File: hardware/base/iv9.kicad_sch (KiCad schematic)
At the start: 0 parts

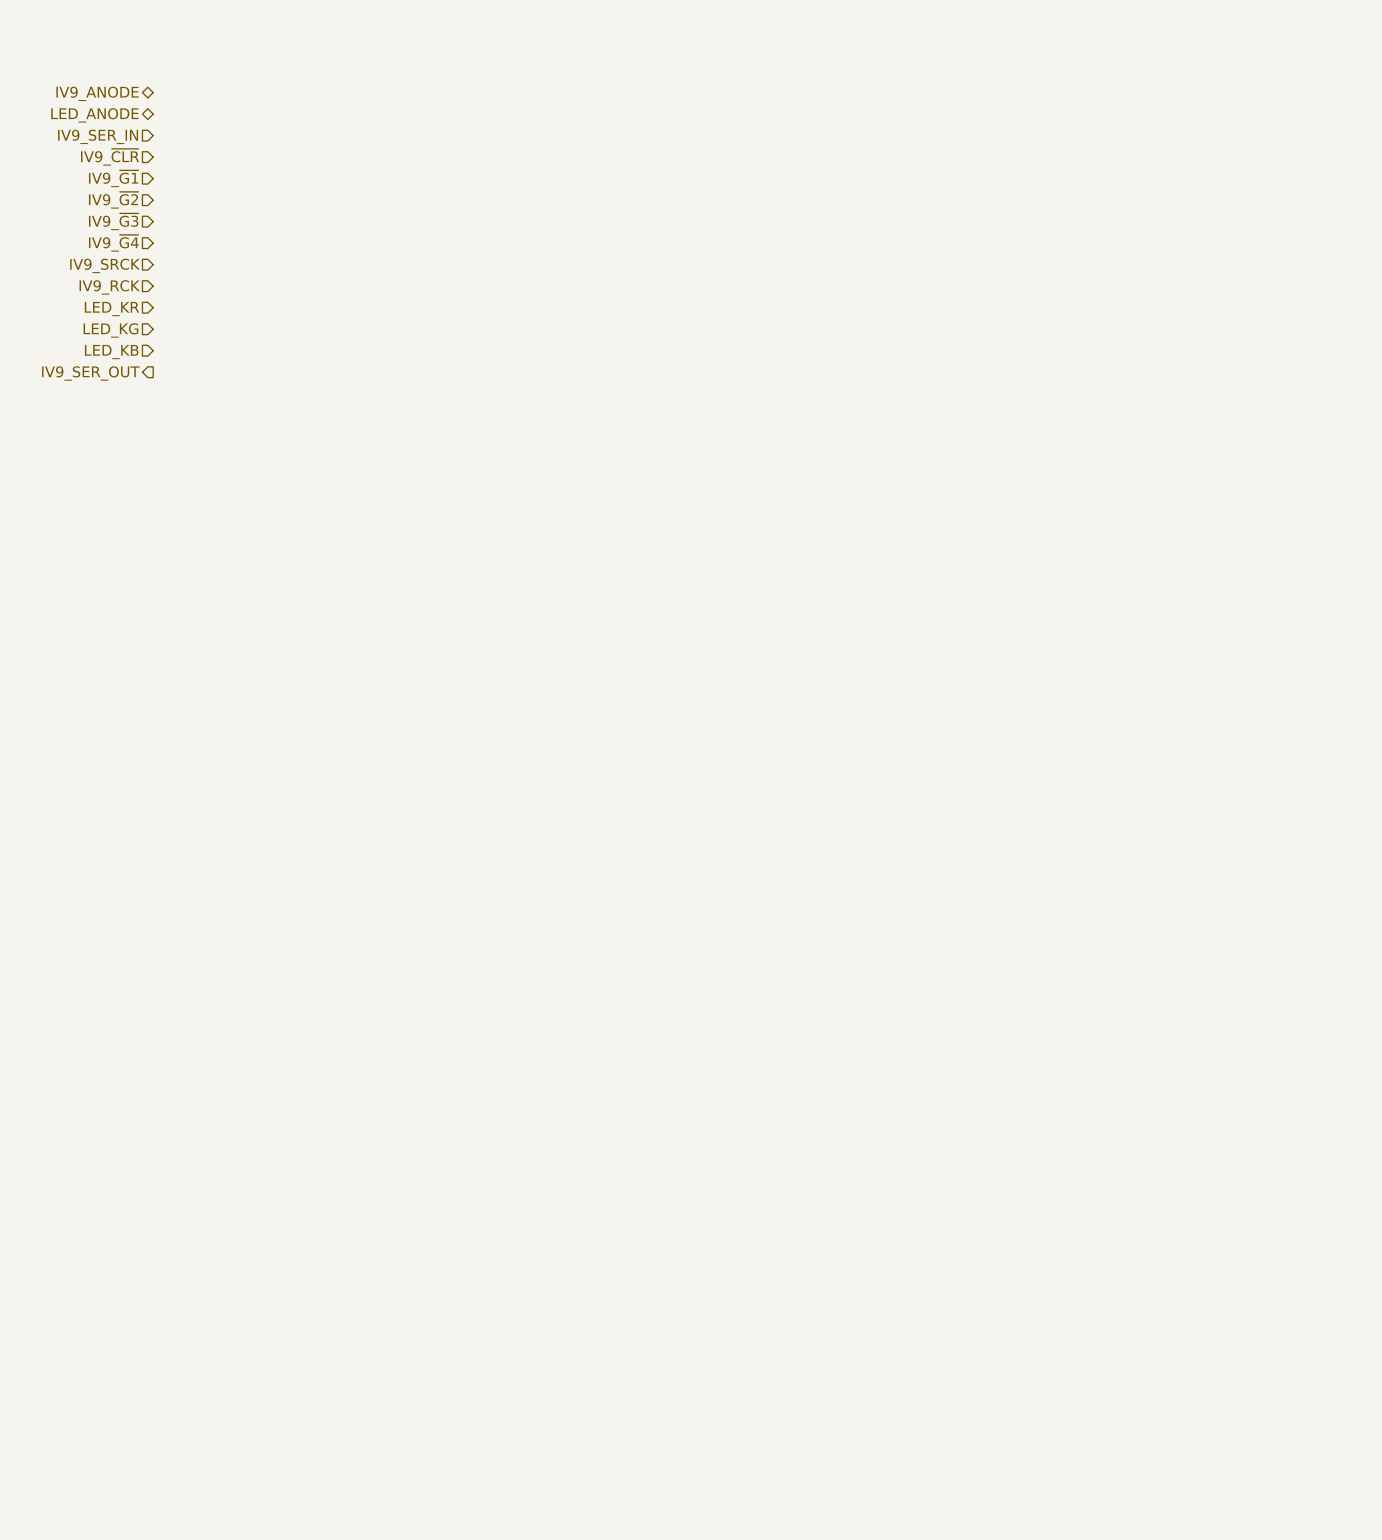
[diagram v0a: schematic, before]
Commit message: Base PCB WIP
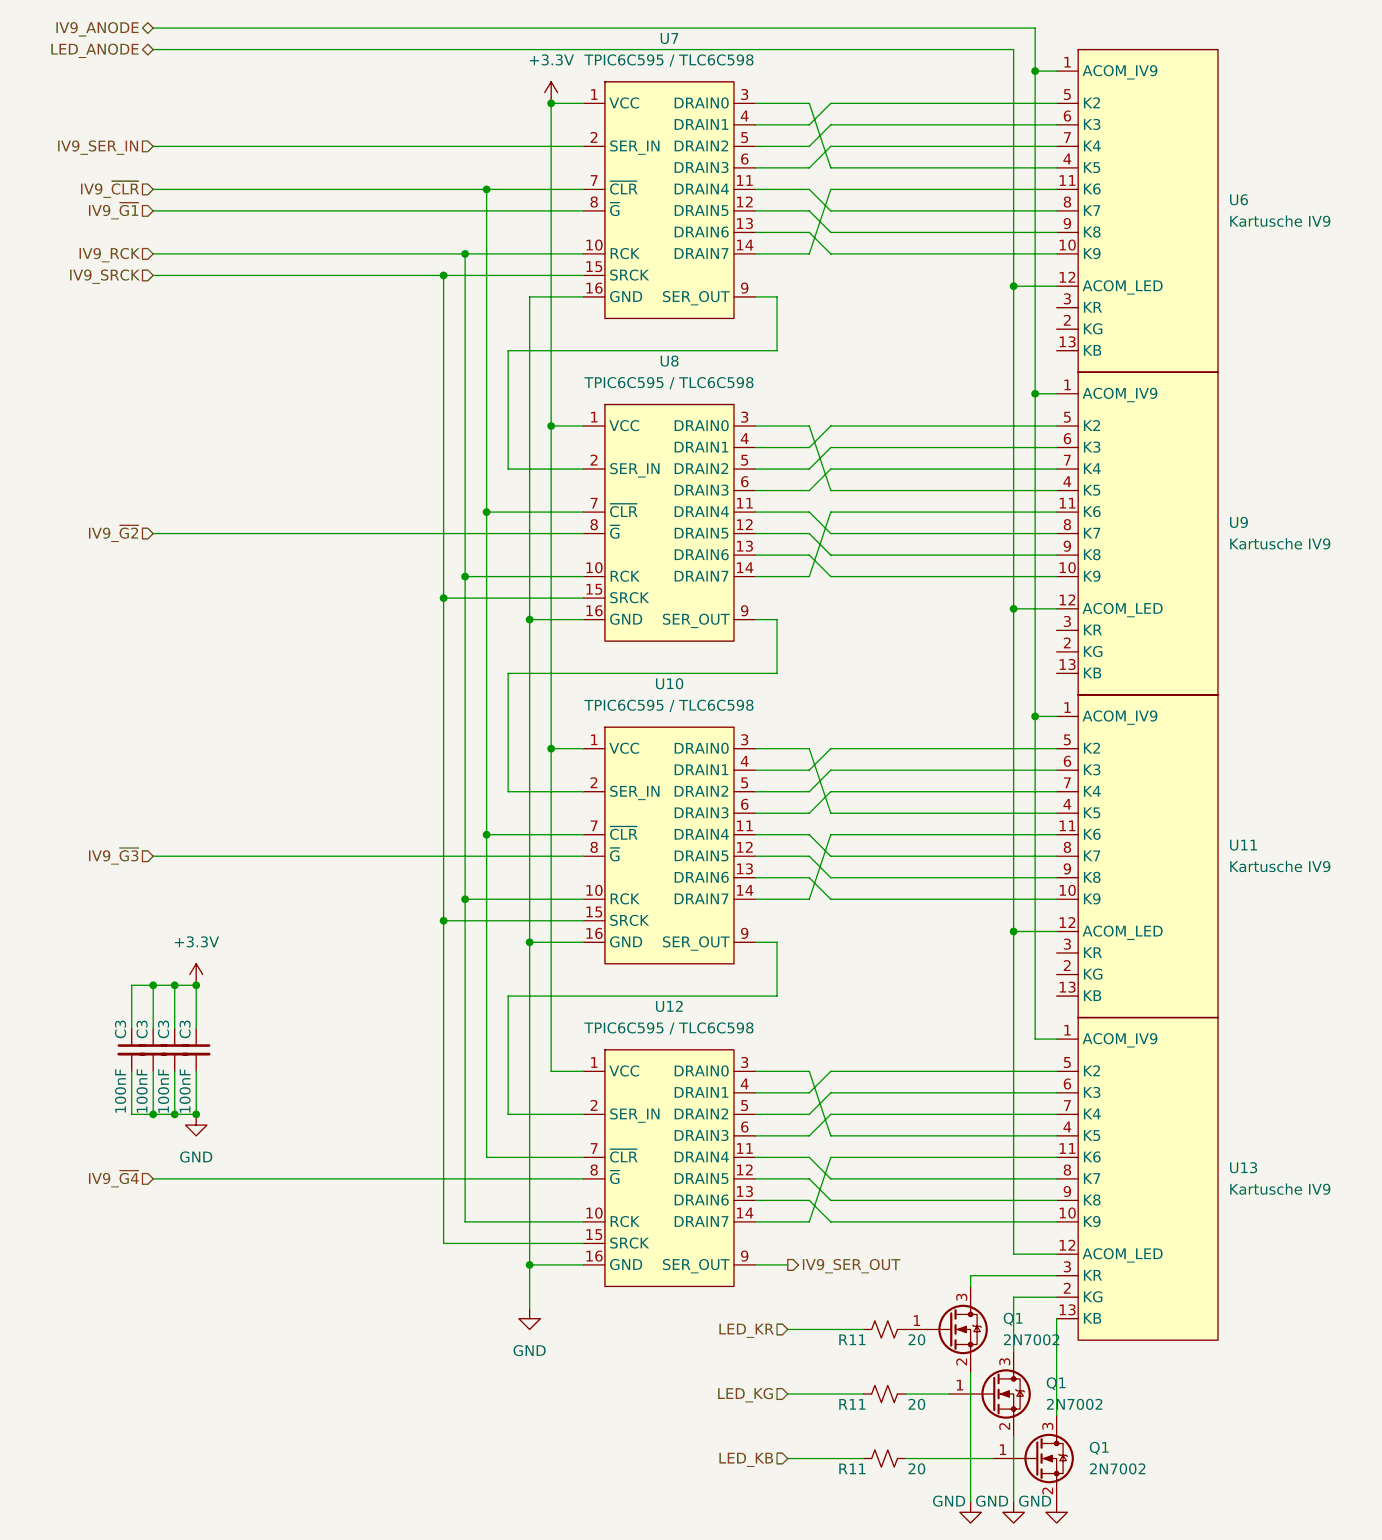
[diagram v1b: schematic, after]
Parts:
- added C3 (x4): 100nF, Capacitor_SMD:C_0402_1005Metric_Pad0.74x0.62mm_HandSolder, symbol Device:C_Small
- added Q1 (x3): 2N7002, Package_TO_SOT_SMD:SOT-23, symbol Transistor_FET:2N7002
- added R11 (x3): 20, Resistor_SMD:R_0402_1005Metric, symbol Device:R_Small_US
- added U10, U12, U7, U8: TPIC6C595 / TLC6C598, Package_SO:SOIC-16_3.9x9.9mm_P1.27mm, symbol Flora:TPIC6C595
- added U11, U13, U6, U9: Kartusche IV9, Flora:Kartusche_IV9, symbol Flora:Kartusche_IV9
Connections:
- net IV9_ANODE: now also U11.1 (ACOM_IV9), U11.14 (ACOM_IV9), U13.1 (ACOM_IV9), U13.14 (ACOM_IV9), U6.1 (ACOM_IV9), U6.14 (ACOM_IV9), U9.1 (ACOM_IV9), U9.14 (ACOM_IV9)
- net IV9_RCK: now also U10.10 (RCK), U12.10 (RCK), U7.10 (RCK), U8.10 (RCK)
- net IV9_SER_IN: now also U7.2 (SER_IN)
- net IV9_SER_OUT: now also U12.9 (SER_OUT)
- net IV9_SRCK: now also U10.15 (SRCK), U12.15 (SRCK), U7.15 (SRCK), U8.15 (SRCK)
- net IV9_~{CLR}: now also U10.7 (~{CLR}), U12.7 (~{CLR}), U7.7 (~{CLR}), U8.7 (~{CLR})
- net IV9_~{G1}: now also U7.8 (~{G})
- net IV9_~{G2}: now also U8.8 (~{G})
- net IV9_~{G3}: now also U10.8 (~{G})
- net IV9_~{G4}: now also U12.8 (~{G})
- net LED_ANODE: now also U11.12 (ACOM_LED), U13.12 (ACOM_LED), U6.12 (ACOM_LED), U9.12 (ACOM_LED)
- net LED_KB: now also R11.1
- net LED_KG: now also R11.1
- net LED_KR: now also R11.1
- new net: Q1.1 (G), R11.2 (x3)
- new net: U6.10 (K9), U7.13 (DRAIN6)
- new net: U6.11 (K6), U7.14 (DRAIN7)
- new net: U6.4 (K5), U7.3 (DRAIN0)
- new net: U6.5 (K2), U7.4 (DRAIN1)
- new net: U6.6 (K3), U7.5 (DRAIN2)
- new net: U6.7 (K4), U7.6 (DRAIN3)
- new net: U6.8 (K7), U7.11 (DRAIN4)
- new net: U6.9 (K8), U7.12 (DRAIN5)
- new net: U10.13 (DRAIN6), U11.10 (K9)
- new net: U10.14 (DRAIN7), U11.11 (K6)
- new net: U10.3 (DRAIN0), U11.4 (K5)
- new net: U10.4 (DRAIN1), U11.5 (K2)
- new net: U10.5 (DRAIN2), U11.6 (K3)
- new net: U10.6 (DRAIN3), U11.7 (K4)
- new net: U10.11 (DRAIN4), U11.8 (K7)
- new net: U10.12 (DRAIN5), U11.9 (K8)
- new net: Q1.3 (D), U13.2 (KG)
- new net: U10.2 (SER_IN), U8.9 (SER_OUT)
- new net: U10.9 (SER_OUT), U12.2 (SER_IN)
- new net: Q1.3 (D), U13.3 (KR)
- new net: U12.13 (DRAIN6), U13.10 (K9)
- new net: U12.14 (DRAIN7), U13.11 (K6)
- new net: Q1.3 (D), U13.13 (KB)
- new net: U12.3 (DRAIN0), U13.4 (K5)
- new net: U12.4 (DRAIN1), U13.5 (K2)
- new net: U12.5 (DRAIN2), U13.6 (K3)
- new net: U12.6 (DRAIN3), U13.7 (K4)
- new net: U12.11 (DRAIN4), U13.8 (K7)
- new net: U12.12 (DRAIN5), U13.9 (K8)
- new net: U7.9 (SER_OUT), U8.2 (SER_IN)
- new net: U8.13 (DRAIN6), U9.10 (K9)
- new net: U8.14 (DRAIN7), U9.11 (K6)
- new net: U8.3 (DRAIN0), U9.4 (K5)
- new net: U8.4 (DRAIN1), U9.5 (K2)
- new net: U8.5 (DRAIN2), U9.6 (K3)
- new net: U8.6 (DRAIN3), U9.7 (K4)
- new net: U8.11 (DRAIN4), U9.8 (K7)
- new net: U8.12 (DRAIN5), U9.9 (K8)
- new net +3.3V: C3.1, C3.1, C3.1, C3.1, U10.1 (VCC), U12.1 (VCC), U7.1 (VCC), U8.1 (VCC)
- new net GND: C3.2, C3.2, C3.2, C3.2, Q1.2 (S), Q1.2 (S), Q1.2 (S), U10.16 (GND), U12.16 (GND), U7.16 (GND), U8.16 (GND)

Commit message: Minor
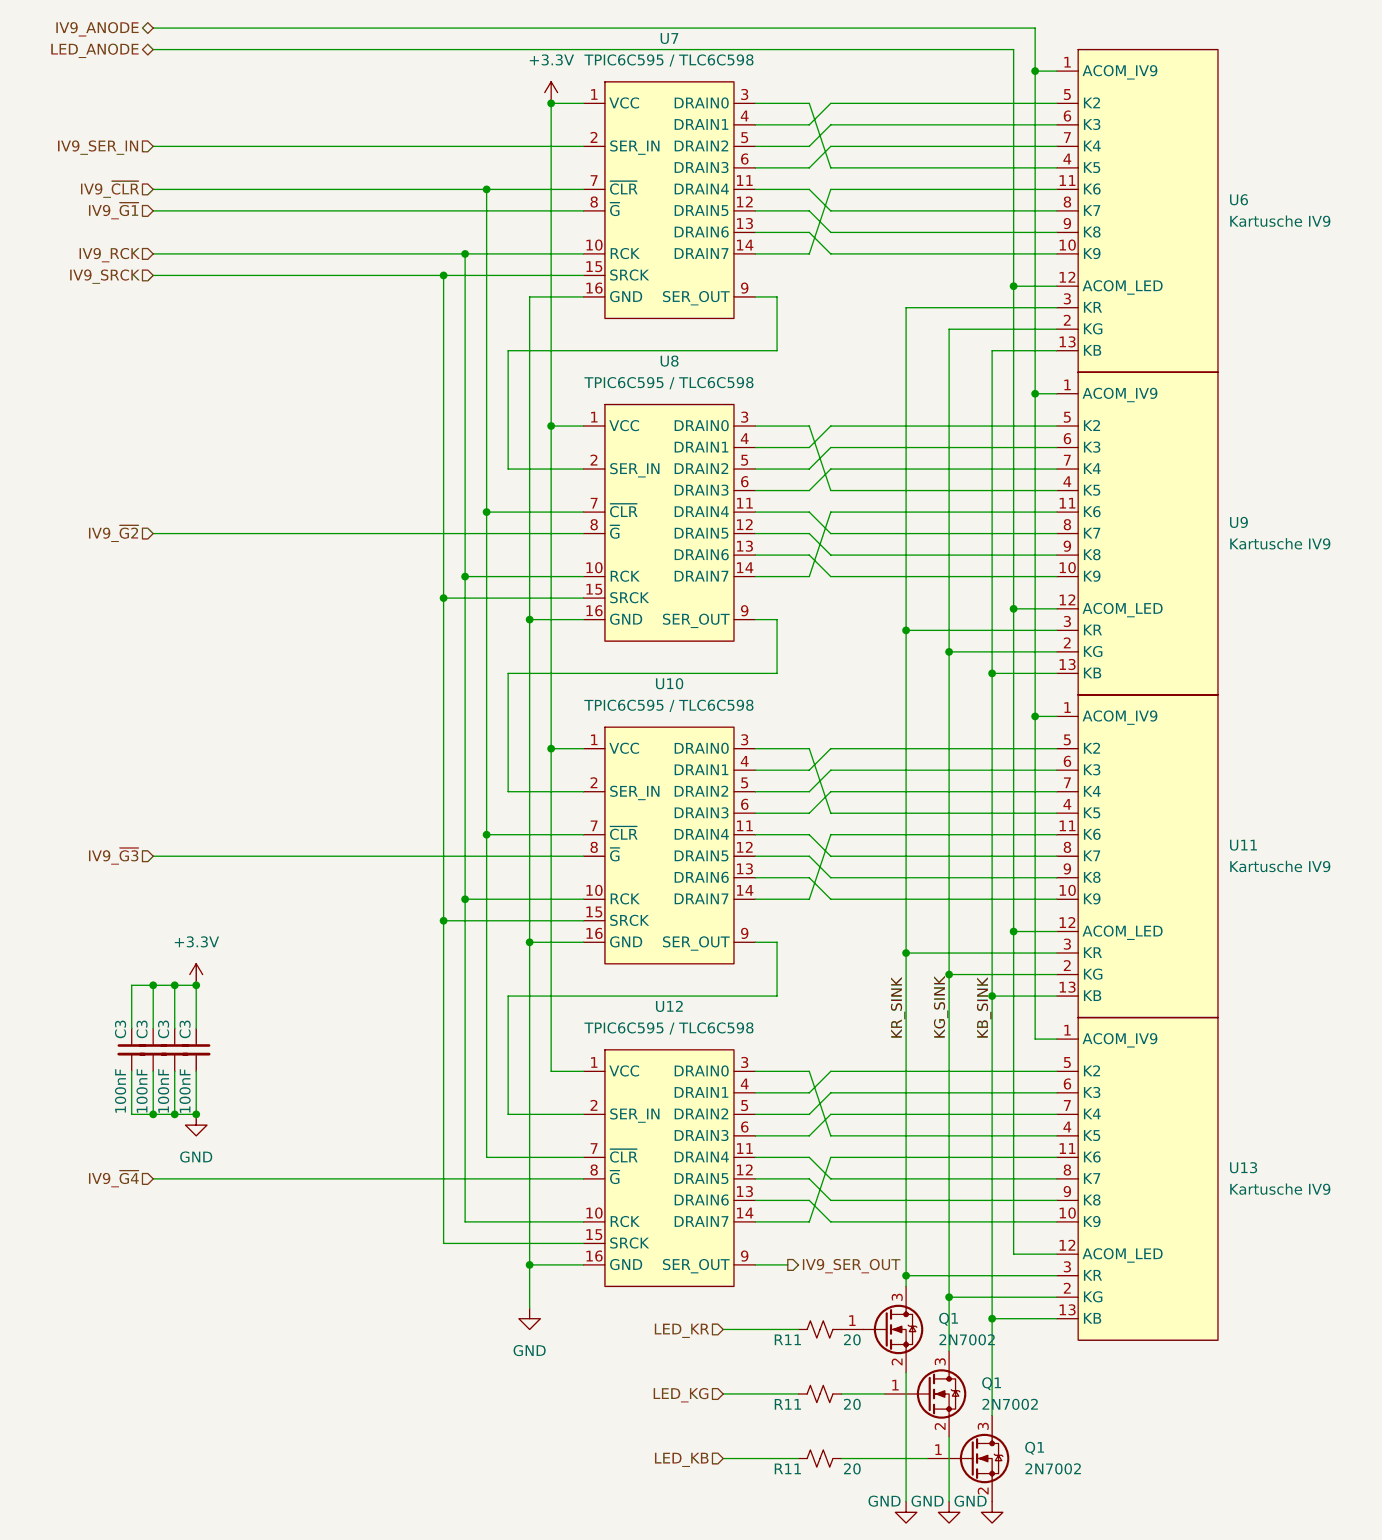
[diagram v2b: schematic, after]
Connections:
- net KB_SINK: now reaches U6.13 (KB)
- net KB_SINK: now also Q1.3 (D), U11.13 (KB), U13.13 (KB), U9.13 (KB)
- net KG_SINK: now reaches U6.2 (KG)
- net KG_SINK: now also Q1.3 (D), U11.2 (KG), U13.2 (KG), U9.2 (KG)
- net KR_SINK: now reaches U6.3 (KR)
- net KR_SINK: now also Q1.3 (D), U11.3 (KR), U13.3 (KR), U9.3 (KR)
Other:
- moved on the sheet: Q1, R11
